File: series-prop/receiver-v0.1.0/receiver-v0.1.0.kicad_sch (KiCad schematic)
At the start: 65 parts, among them IC1 LM66200DRLR, J1 Conn_01x17, J10 Conn_01x03_Pin, J11 Conn_01x04_Pin, J13 USB_C_Receptacle_USB2.0_16P, J2 Conn_01x04_Pin, J4 Conn_01x17, J5 Conn_01x01_Pin, J6 Screw_Terminal_01x02, J7 Screw_Terminal_01x03, J8 Conn_Coaxial, J9 SM04B-SRSS-TB, SW1 SW_Push, SW2 SW_Push, SW3 SW_Push, SW4 SW_Push, U1 RT9080-33GJ5, U2 W25Q16JVS, U3 RP2040, U4 RFM69HCW, U5 AP63205WU, U6 74AHCT1G125, U7 3544-2, Y1 Crystal_GND24

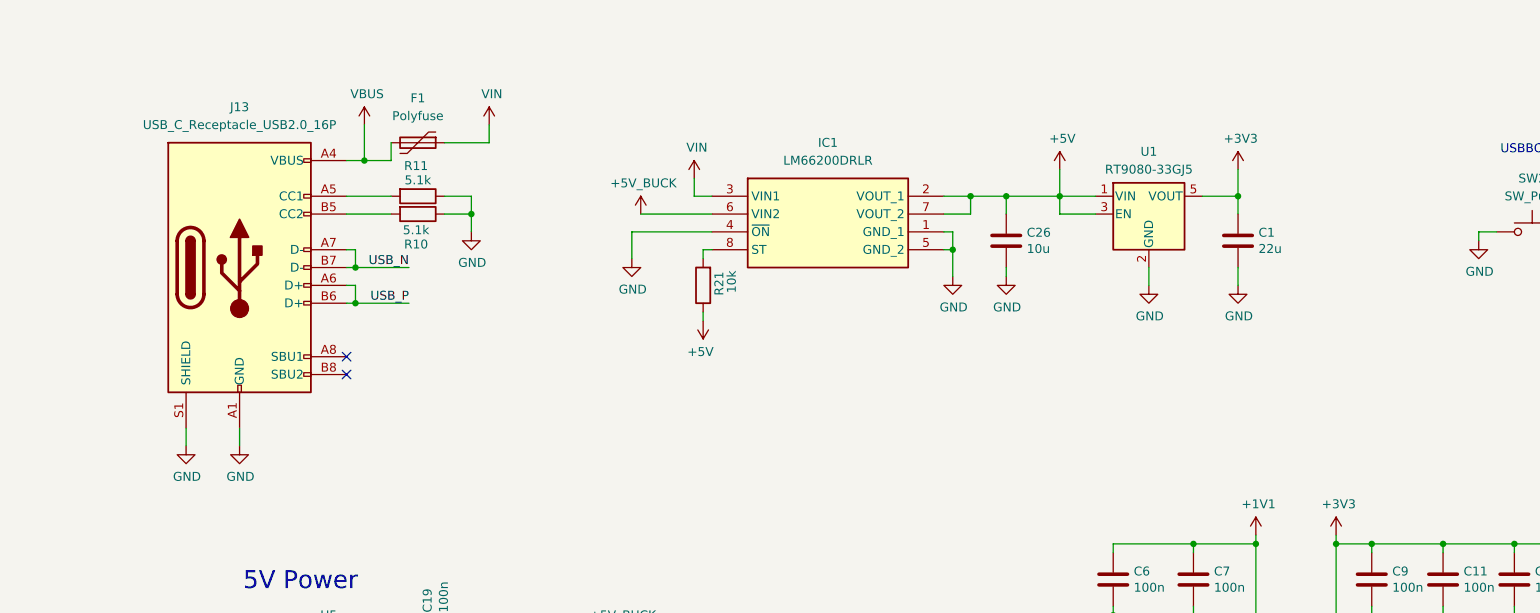
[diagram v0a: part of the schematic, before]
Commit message: added remote design files
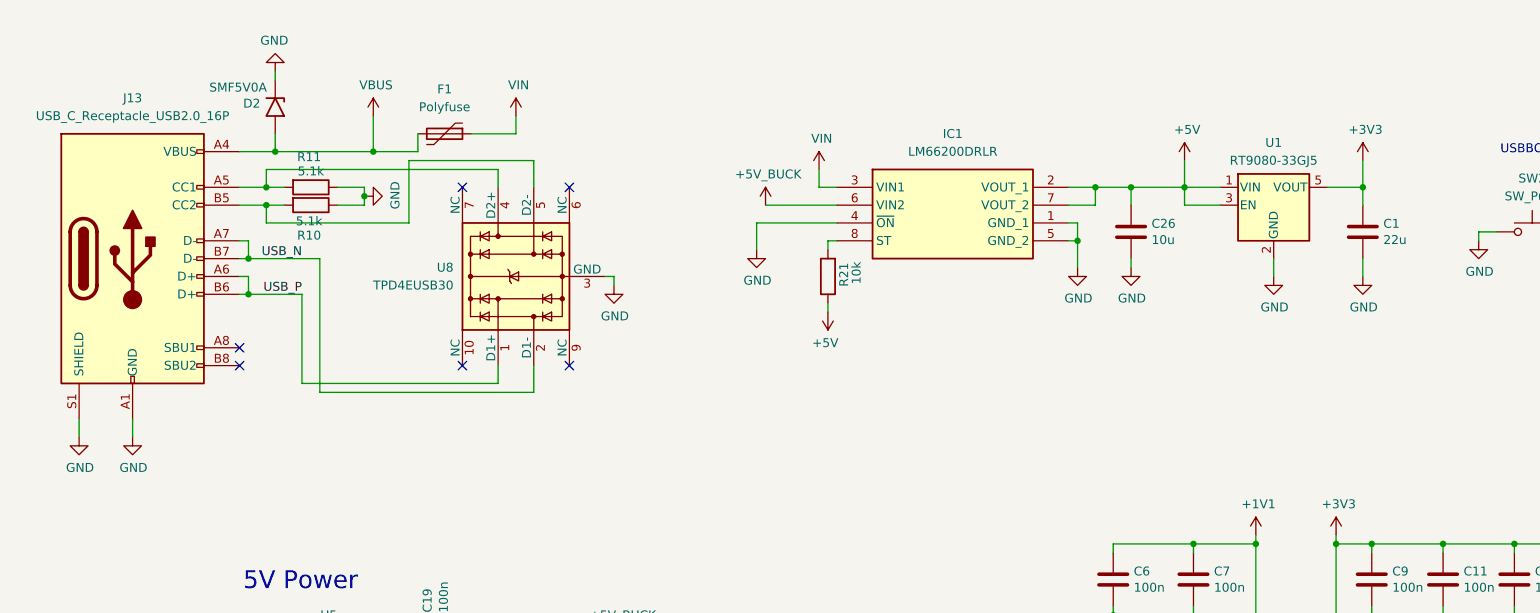
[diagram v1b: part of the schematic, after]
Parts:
- added D2: SMF5V0A, Diode_SMD:D_SMF, symbol Diode:SMF5V0A
- added U8: TPD4EUSB30, Package_SON:USON-10_2.5x1.0mm_P0.5mm, symbol Power_Protection:TPD4EUSB30
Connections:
- net GND: now also D2.1 (A1), U8.3 (GND), U8.8 (GND)
- net USB_N: now also U8.2 (D1-)
- net USB_P: now also U8.1 (D1+)
- net VBUS: now also D2.2 (A2)
- net at J13.B5 (CC2), R10.2: now also U8.5 (D2-)
- net at J13.A5 (CC1), R11.2: now also U8.4 (D2+)
- no-connect marks 4 -> 8
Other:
- moved on the sheet: C1, C26, F1, IC1, J13, R10, R11, R21, U1
